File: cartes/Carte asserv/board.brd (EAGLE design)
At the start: 50.8 x 66 mm, 13 parts, among them X1 MICROMATCH-6, X2 MICROMATCH-6

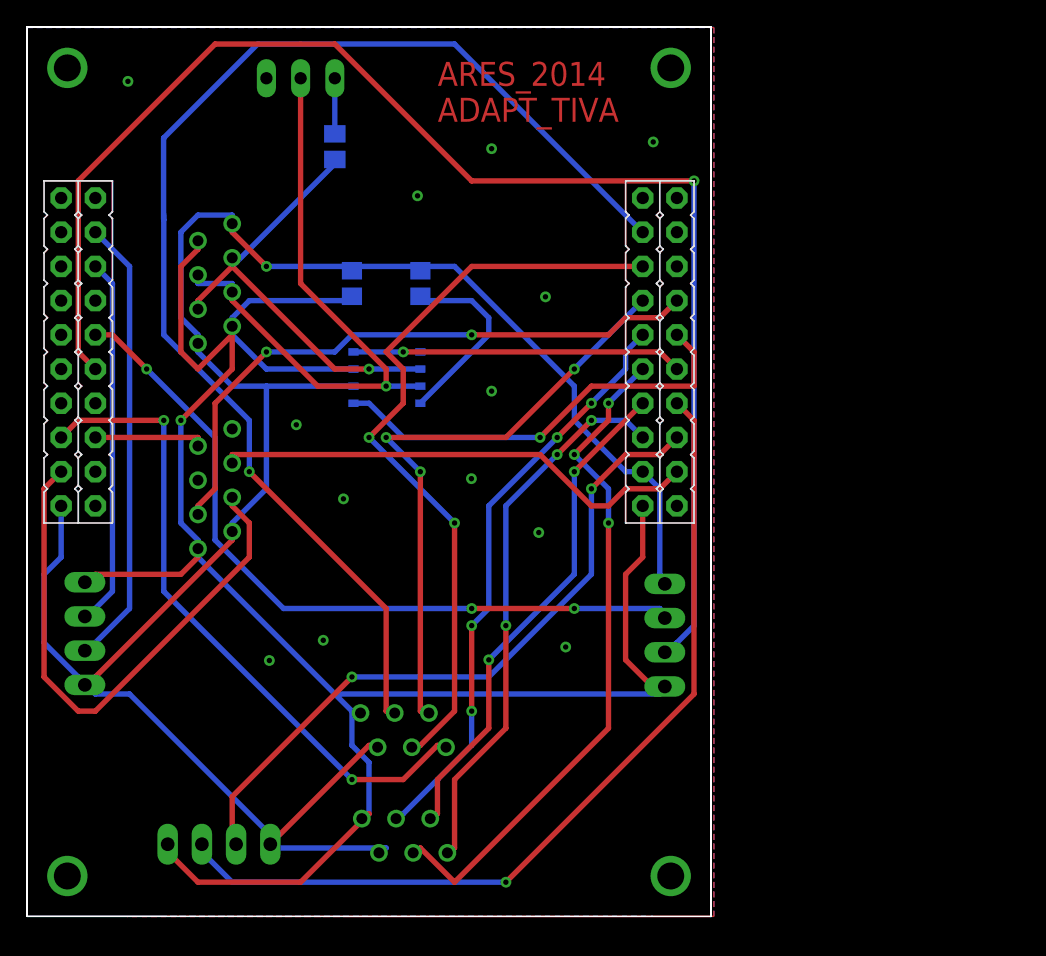
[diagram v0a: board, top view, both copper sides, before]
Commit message: nouvelles cartes à jour
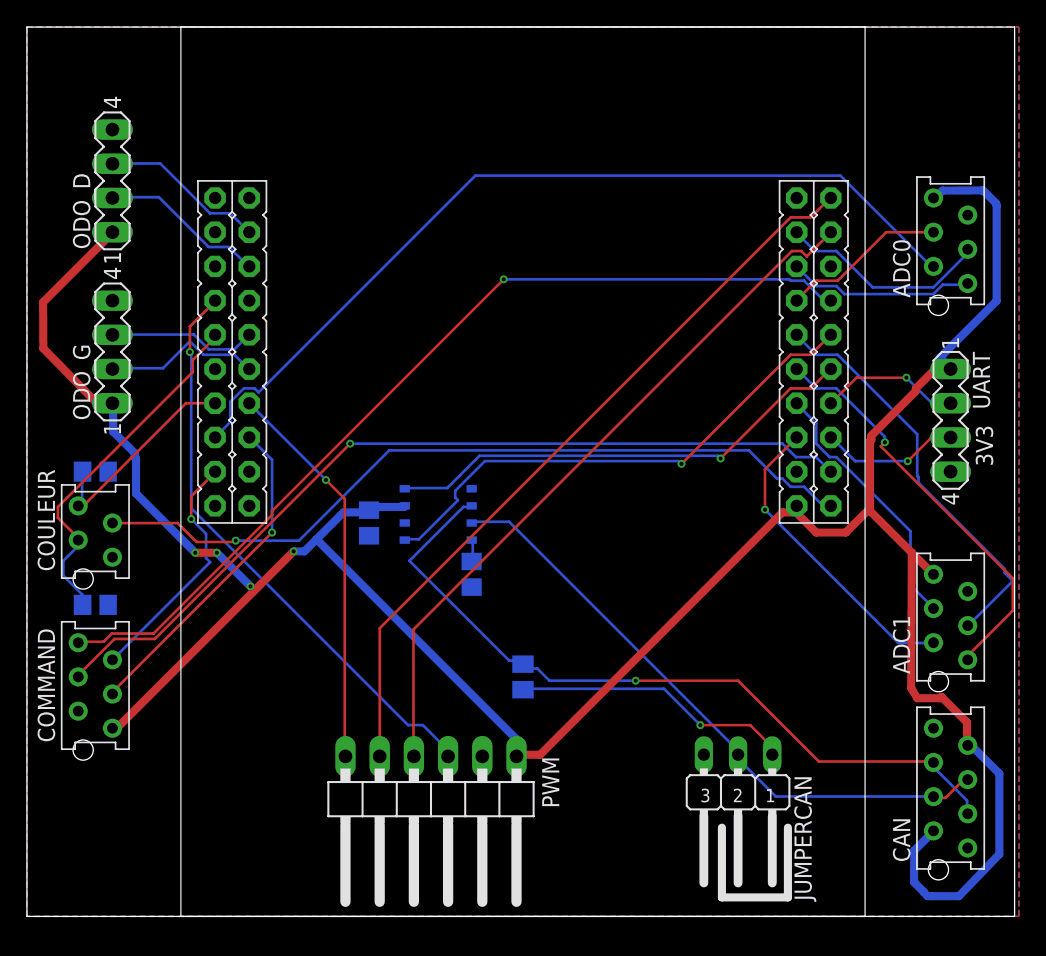
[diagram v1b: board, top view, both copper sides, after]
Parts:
- removed JP1: (no value), jumper:JP2W
- removed X1, X2: MICROMATCH-6, con-amp-micromatch:MICROMATCH-6
- added ADC0, ADC1: MMATCH-6-, jt-con-micromatch:AMP-215079-6
- added COULEUR: MMATCH-4-, jt-con-micromatch:AMP-215079-4
- added JUMPERCAN: (no value), jumper:JP2W
- added PWM: (no value), pinhead:1X06/90
- added R10, R11: 10k, rcl:R0805
- CAN: value MICROMATCH-8 -> (none); device con-amp-micromatch:MICROMATCH-8 -> jt-con-micromatch:AMP-215079-8
- COMMAND: value MICROMATCH-8 -> MMATCH-6-; device con-amp-micromatch:MICROMATCH-8 -> jt-con-micromatch:AMP-215079-6
- moved CAN 68.8 mm to (68.6, 5.08), flipped to the top, turned to 90 degrees
- moved UART 62.8 mm to (68.6, 36.8), flipped to the top, turned to 270 degrees
- moved ODO_G 46.1 mm to (6.35, 41.9), flipped to the top
- moved R5 41.8 mm to (36.8, 17.8), turned to 270 degrees
- moved ODO_D 33.7 mm to (6.35, 54.6), flipped to the top, turned to 90 degrees
- moved R1 21.9 mm to (33.0, 25.4), turned to 270 degrees
- moved COMMAND 19.3 mm to (6.35, 14.0), flipped to the top, turned to 90 degrees
- moved C1 17.8 mm to (25.4, 29.2), turned to 90 degrees
- moved TIVA 11.4 mm to (62.2, 0.00)
- moved U$1 10.9 mm to (33.0, 27.9)
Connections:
- removed net 3.3V: TIVA.3.3V
- removed net TF1: COMMAND.8
- removed net TF2: COMMAND.5
- new net COULEUR: COULEUR.4, R11.2, TIVA.PF0
- new net PWM1: PWM.3, TIVA.PB6
- new net PWM2: PWM.4, TIVA.PA6
- new net PWM3: PWM.5, TIVA.PA7
- new net PWM4: PWM.6, TIVA.PC4
- new net TIRETTE: COULEUR.2, R10.2, TIVA.PB7
- new net VDD_3V3: COULEUR.3, TIVA.3.3V
- net +5V: now also ADC0.6, ADC1.6, PWM.1; no longer X1.1, X2.1
- net ADC_0: now also ADC0.3; no longer X1.3
- net ADC_1: now also ADC0.1; no longer X1.4
- net ADC_2: now also ADC0.4; no longer X1.5
- net ADC_3: now also ADC0.2; no longer X1.6
- net ADC_4: now also ADC1.3; no longer X2.3
- net ADC_5: now also ADC1.1; no longer X2.4
- net ADC_6: now also ADC1.4; no longer X2.5
- net ADC_7: now also ADC1.2; no longer X2.6
- net CANH: now also JUMPERCAN.2; no longer JP1.2
- net DIR1: now also COMMAND.3; no longer COMMAND.7
- net DIR2: now also COMMAND.5; no longer COMMAND.4
- net GND: now also ADC0.5, ADC1.5, COULEUR.1, PWM.2, R10.1, R11.1; no longer X1.2, X2.2
- net N$9: now also JUMPERCAN.1; no longer JP1.1
- net PWM_MOT1: now also COMMAND.4; no longer COMMAND.6
- net PWM_MOT2: now also COMMAND.6; no longer COMMAND.3
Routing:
- net GND: track 160.2 -> 0.00 mm, vias 14 -> 0
- net CHA_G: track 104.6 -> 11.9 mm, vias 1 -> 0
- net ADC_0: track 94.6 -> 15.8 mm, vias 1 -> 0
- net VDD_3V3: track 0.00 -> 58.4 mm, vias 0 -> 1
- net PWM3: track 0.00 -> 56.2 mm
- net UART_TX: track 66.2 -> 10.5 mm
- net PWM2: track 0.00 -> 53.0 mm
- net +5V: track 150.3 -> 202.6 mm, vias 1 -> 4
- net CHB_G: track 55.6 -> 11.1 mm, vias 3 -> 0
- net PWM1: track 0.00 -> 43.3 mm, vias 0 -> 1
- net ADC_1: track 56.8 -> 13.9 mm, vias 2 -> 0
- net UART_RX: track 51.4 -> 10.4 mm, vias 2 -> 1
- net ADC_2: track 45.3 -> 12.3 mm, vias 3 -> 0
- net PWM4: track 0.00 -> 29.2 mm, vias 0 -> 1
- net PWM_MOT1: track 36.3 -> 64.0 mm, vias 0 -> 1
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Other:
- board size 50.8 x 66 mm -> 73.3 x 66 mm
- board text added: "3V3"
- board text removed: "ADC"
- board text removed: "ARES_2014 ADAPT_TIVA"
- board text removed: "CAN"
- board text removed: "COMMAND"
- board text removed: "JUMPER CAN"
- board text removed: "ODO_D"
- board text removed: "ODO_G"
- board text removed: "UART"
